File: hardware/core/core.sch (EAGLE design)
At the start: 529 parts, among them IC1 MAX481CSA, IC10 MAX481CSA, IC11 MAX481CSA, IC12 MAX481CSA, IC13 MAX481CSA, IC14 MAX481CSA, IC15 MAX481CSA, IC16 MAX481CSA, IC17 MAX481CSA, IC18 MAX481CSA, IC19 MAX481CSA, IC2 LD117AS12TR, IC20 MAX481CSA, IC21 MAX481CSA, IC22 LD117AS12TR, IC23 LD117AS12TR, IC3 MAX481CSA, IC4 MAX481CSA, IC5 MAX481CSA, IC6 MAX481CSA, IC7 MAX481CSA, IC8 MAX481CSA, IC9 MAX481CSA

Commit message: Update phoenix connectors & add JLC_ROTATION
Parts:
- added D100, D101, D102, D103, D104, D105, D106, D107, D108, D109, D110, D111, D112, D113, D114, D95, D96, D97, D98, D99: D_B5819W-SL_CHANGJ_SOD123, JLC PCB Basic Parts_loc:D_B5819W-SL_CHANGJ_SOD123
- POWER_IN: device con-phoenix-508:MKDSN1,5/4-5,08 -> con-phoenix-508-jm:MKDSN1,5/4-5,08
- R132: value R_1.8K_0603 -> R_1K_0603; device JLC PCB Basic Parts_loc:R_1.8K_0603 -> JLC PCB Basic Parts_loc:R_1K_0603
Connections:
- new net N$325: D95.C, STAR_1.6
- new net N$326: D97.C, STAR_3.6
- new net N$327: D96.A, R55.2
- new net N$328: D96.C, STAR_2.6
- new net N$329: D100.A, R59.2
- new net N$330: D100.C, STAR_6.6
- new net N$331: D99.A, R58.2
- new net N$332: D99.C, STAR_5.6
- new net N$333: D110.A, R85.2
- new net N$334: D110.C, STAR_15.6
- new net N$335: D109.A, R84.2
- new net N$336: D109.C, STAR_14.6
- new net N$337: D105.A, R103.2
- new net N$338: D105.C, STAR_17.6
- new net N$339: D112.A, R104.2
- new net N$340: D112.C, STAR_18.6
- new net N$341: D113.A, R105.2
- new net N$342: D113.C, STAR_19.6
- new net N$343: D114.A, R106.2
- new net N$344: D114.C, STAR_20.6
- net N$10: now also D102.A, R61.2; no longer R58.2, STAR_5.6
- net N$104: now also D108.A, R65.2; no longer R104.2, STAR_18.6
- net N$105: now also D108.C, STAR_12.6; no longer R105.2, STAR_19.6
- net N$106: now also D111.A, R86.2; no longer R106.2, STAR_20.6
- net N$107: now also D111.C, STAR_16.6; no longer R103.2, STAR_17.6
- net N$15: now also D102.C, STAR_8.6; no longer R59.2, STAR_6.6
- net N$16: now also D101.A; no longer STAR_7.6
- net N$17: now also D101.C, STAR_7.6; no longer R61.2, STAR_8.6
- net N$18: now also D103.A, R62.2; no longer R65.2, STAR_12.6
- net N$19: now also D103.C, STAR_9.6; no longer R64.2, STAR_11.6
- net N$2: now also D98.A, R57.2; no longer R55.2, STAR_2.6
- net N$24: now also D104.A, R83.2; no longer R63.2, STAR_10.6
- net N$25: now also D104.C, STAR_13.6; no longer R62.2, STAR_9.6
- net N$7: now also D98.C, STAR_4.6; no longer R56.2, STAR_3.6
- net N$72: now also D106.A, R63.2; no longer R84.2, STAR_14.6
- net N$73: now also D106.C, STAR_10.6; no longer R85.2, STAR_15.6
- net N$74: now also D107.A, R64.2; no longer R86.2, STAR_16.6
- net N$75: now also D107.C, STAR_11.6; no longer R83.2, STAR_13.6
- net N$8: now also D97.A, R56.2; no longer R57.2, STAR_4.6
- net N$9: now also D95.A; no longer STAR_1.6

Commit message: Replaced output resistor with 68 ohm (part c27592)
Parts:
- R103, R104, R105, R106, R140, R141, R142, R143, R144, R145, R146, R147, R148, R149, R150, R151, R152, R153, R154, R155, R156, R157, R158, R159, R160, R161, R162, R163, R164, R165, R166, R167, R168, R169, R170, R171, R172, R173, R174, R175, R176, R177, R178, R179, R180, R181, R182, R183, R184, R185, R186, R187, R188, R189, R190, R191, R192, R193, R194, R195, R196, R197, R198, R199, R200, R201, R202, R203, R204, R205, R206, R207, R208, R209, R210, R211, R212, R213, R214, R215, R216, R217, R218, R219, R54, R55, R56, R57, R58, R59, R60, R61, R62, R63, R64, R65, R83, R84, R85, R86: LCSC_PART C25804 -> c27592

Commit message: Add TVS and change led resistors to 1k
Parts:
- removed I2C_1: (no value), pinhead:PINHD-1X4
- removed ULN10, ULN11, ULN12, ULN3, ULN4, ULN5, ULN6, ULN7, ULN8, ULN9: (no value), SparkFun-IC-Special-Function:ULN2803SOICW
- added D115, D116, D117, D118, D119, D120, D121, D122, D123, D124, D125, D126, D127, D128, D129, D130, D131, D132, D133, D134, D135, D136, D137, D138, D139, D140, D141, D142, D143, D144, D145, D146, D147, D148, D149, D150, D151, D152, D153, D154, D155, D156, D157, D158, D159, D160, D161, D162, D163, D164, D165, D166, D167, D168, D169, D170, D171, D172, D173, D174, D175, D176, D177, D178, D179, D180, D181, D182, D183, D184, D185, D186, D187, D188, D189, D190, D191, D192, D193, D194, D195: SMBJ8.0CA, SMBJ8.0CA:SMBJ8.0CA
- added R226, R227, R228, R229, R230, R231, R232, R233, R234, R235, R236, R237, R238, R239, R240, R241, R242, R243, R244, R245, R246, R247, R248, R249, R250, R251, R252, R253, R254, R255, R256, R257, R258, R259, R260, R261, R262, R263, R264, R265, R266, R267, R268, R269, R270, R271, R272, R273, R274, R275, R276, R277, R278, R279, R280, R281, R282, R283, R284, R285, R286, R287, R288, R289, R290, R291, R292, R293, R294, R295, R296, R297, R298, R299, R300, R301, R302, R303, R304, R305: 68, rcl:R-US_R0603
- R10, R100, R101, R102, R11, R12, R13, R14, R15, R16, R17, R18, R19, R20, R21, R22, R23, R24, R25, R28, R29, R3, R30, R31, R32, R33, R34, R35, R36, R37, R38, R39, R4, R40, R41, R42, R43, R44, R45, R46, R47, R48, R49, R5, R50, R51, R52, R53, R6, R66, R69, R7, R70, R71, R72, R73, R74, R75, R76, R77, R78, R79, R8, R80, R81, R82, R87, R88, R89, R9, R90, R91, R92, R93, R94, R95, R96, R97, R98, R99: value 10k -> 1k; LCSC_PART C25804 -> C21190
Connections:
- new net N$345: C45.1, D123.2, R11.1, R151.1, R234.2
- net +12V: no longer ULN10.10, ULN11.10, ULN12.10, ULN3.10, ULN4.10, ULN5.10, ULN6.10, ULN7.10, ULN8.10, ULN9.10
- net +3V3: no longer I2C_1.1
- net +5V: no longer D1.A, D10.A, D11.A, D12.A, D13.A, D14.A, D15.A, D16.A, D17.A, D18.A, D19.A, D2.A, D20.A, D21.A, D22.A, D23.A, D24.A, D25.A, D26.A, D27.A, D28.A, D29.A, D3.A, D30.A, D31.A, D32.A, D33.A, D34.A, D35.A, D36.A, D37.A, D38.A, D39.A, D4.A, D40.A, D41.A, D42.A, D43.A, D44.A, D45.A, D46.A, D47.A, D48.A, D49.A, D5.A, D50.A, D51.A, D52.A, D53.A, D54.A, D55.A, D56.A, D57.A, D58.A, D59.A, D6.A, D60.A, D61.A, D62.A, D63.A, D64.A, D65.A, D66.A, D67.A, D68.A, D69.A, D7.A, D70.A, D71.A, D72.A, D73.A, D74.A, D75.A, D76.A, D77.A, D78.A, D79.A, D8.A, D80.A, D9.A
- net 21/SDA: no longer I2C_1.4
- net 22/SCL: no longer I2C_1.3
- net A0: now also R226.1; no longer ULN3.8
- net A1: now also R227.1; no longer ULN3.7
- net A10: now also R236.1; no longer ULN4.6
- net A11: now also R237.1; no longer ULN4.5
- net A12: now also R238.1; no longer ULN4.4
- net A13: now also R239.1; no longer ULN4.3
- net A14: now also R240.1; no longer ULN4.2
- net A15: now also R241.1; no longer ULN4.1
- net A2: now also R228.1; no longer ULN3.6
- net A3: now also R229.1; no longer ULN3.5
- net A4: now also R230.1; no longer ULN3.4
- net A5: now also R231.1; no longer ULN3.3
- net A6: now also R232.1; no longer ULN3.2
- net A7: now also R233.1; no longer ULN3.1
- net A8: now also R234.1; no longer ULN4.8
- net A9: now also R235.1; no longer ULN4.7
- net B0: now also R242.1; no longer ULN5.8
- net B1: now also R243.1; no longer ULN5.7
- net B10: now also R252.1; no longer ULN6.6
- net B11: now also R253.1; no longer ULN6.5
- net B12: now also R254.1; no longer ULN6.4
- net B13: now also R255.1; no longer ULN6.3
- net B14: now also R256.1; no longer ULN6.2
- net B15: now also R257.1; no longer ULN6.1
- net B2: now also R244.1; no longer ULN5.6
- net B3: now also R245.1; no longer ULN5.5
- net B4: now also R246.1; no longer ULN5.4
- net B5: now also R247.1; no longer ULN5.3
- net B6: now also R248.1; no longer ULN5.2
- net B7: now also R249.1; no longer ULN5.1
- net B8: now also R250.1; no longer ULN6.8
- net B9: now also R251.1; no longer ULN6.7
- net C0: now also R258.1; no longer ULN7.8
- net C1: now also R259.1; no longer ULN7.7
- net C10: now also R268.1; no longer ULN8.6
- net C11: now also R269.1; no longer ULN8.5
- net C12: now also R270.1; no longer ULN8.4
- net C13: now also R271.1; no longer ULN8.3
- net C14: now also R272.1; no longer ULN8.2
- net C15: now also R273.1; no longer ULN8.1
- net C2: now also R260.1; no longer ULN7.6
- net C3: now also R261.1; no longer ULN7.5
- net C4: now also R262.1; no longer ULN7.4
- net C5: now also R263.1; no longer ULN7.3
- net C6: now also R264.1; no longer ULN7.2
- net C7: now also R265.1; no longer ULN7.1
- net C8: now also R266.1; no longer ULN8.8
- net C9: now also R267.1; no longer ULN8.7
- net D0: now also R274.1; no longer ULN9.8
- net D1: now also R275.1; no longer ULN9.7
- net D10: now also R284.1; no longer ULN10.6
- net D11: now also R285.1; no longer ULN10.5
- net D12: now also R286.1; no longer ULN10.4
- net D13: now also R287.1; no longer ULN10.3
- net D14: now also R288.1; no longer ULN10.2
- net D15: now also R289.1; no longer ULN10.1
- net D2: now also R276.1; no longer ULN9.6
- net D3: now also R277.1; no longer ULN9.5
- net D4: now also R278.1; no longer ULN9.4
- net D5: now also R279.1; no longer ULN9.3
- net D6: now also R280.1; no longer ULN9.2
- net D7: now also R281.1; no longer ULN9.1
- net D8: now also R282.1; no longer ULN10.8
- net D9: now also R283.1; no longer ULN10.7
- net E0: now also R290.1; no longer ULN11.8
- net E1: now also R291.1; no longer ULN11.7
- net E10: now also R300.1; no longer ULN12.6
- net E11: now also R301.1; no longer ULN12.5
- net E12: now also R302.1; no longer ULN12.4
- net E13: now also R303.1; no longer ULN12.3
- net E14: now also R304.1; no longer ULN12.2
- net E15: now also R305.1; no longer ULN12.1
- net E2: now also R292.1; no longer ULN11.6
- net E3: now also R293.1; no longer ULN11.5
- net E4: now also R294.1; no longer ULN11.4
- net E5: now also R295.1; no longer ULN11.3
- net E6: now also R296.1; no longer ULN11.2
- net E7: now also R297.1; no longer ULN11.1
- net E8: now also R298.1; no longer ULN12.8
- net E9: now also R299.1; no longer ULN12.7
- net GND: now also D10.C, D11.C, D115.1, D116.1, D117.1, D118.1, D119.1, D12.C, D120.1, D121.1, D122.1, D123.1, D124.1, D125.1, D126.1, D127.1, D128.1, D129.1, D13.C, D130.1, D131.1, D132.1, D133.1, D134.1, D135.1, D136.1, D137.1, D138.1, D139.1, D14.C, D140.1, D141.1, D142.1, D143.1, D144.1, D145.1, D146.1, D147.1, D148.1, D149.1, D15.C, D150.1, D151.1, D152.1, D153.1, D154.1, D155.1, D156.1, D157.1, D158.1, D159.1, D16.C, D160.1, D161.1, D162.1, D163.1, D164.1, D165.1, D166.1, D167.1, D168.1, D169.1, D17.C, D170.1, D171.1, D172.1, D173.1, D174.1, D175.1, D176.1, D177.1, D178.1, D179.1, D18.C, D180.1, D181.1, D182.1, D183.1, D184.1, D185.1, D186.1, D187.1, D188.1, D189.1, D19.C, D190.1, D191.1, D192.1, D193.1, D194.1, D195.1, D2.C, D20.C, D21.C, D22.C, D23.C, D24.C, D25.C, D26.C, D27.C, D28.C, D29.C, D3.C, D30.C, D31.C, D32.C, D33.C, D34.C, D35.C, D36.C, D37.C, D38.C, D39.C, D4.C, D40.C, D41.C, D42.C, D43.C, D44.C, D45.C, D46.C, D47.C, D48.C, D49.C, D5.C, D57.C, D58.C, D59.C, D6.C, D60.C, D61.C, D62.C, D63.C, D64.C, D65.C, D66.C, D67.C, D68.C, D69.C, D7.C, D70.C, D71.C, D72.C, D73.C, D74.C, D75.C, D76.C, D77.C, D78.C, D79.C, D8.C, D80.C, D9.C; no longer I2C_1.2, ULN10.9, ULN11.9, ULN12.9, ULN3.9, ULN4.9, ULN5.9, ULN6.9, ULN7.9, ULN8.9, ULN9.9
- net N$100: now also D69.A, R91.2; no longer D77.C, R99.2
- net N$101: now also D70.A, R92.2; no longer D78.C, R100.2
- net N$102: now also D71.A, R93.2; no longer D79.C, R101.2
- net N$103: now also D72.A, R94.2; no longer D80.C, R102.2
- net N$11: now also D6.A; no longer D6.C
- net N$12: now also D7.A; no longer D7.C
- net N$13: now also D8.A; no longer D8.C
- net N$14: now also D9.A; no longer D9.C
- net N$160: now also D116.2, R226.2; no longer ULN3.11
- net N$161: now also D115.2, R227.2; no longer ULN3.12
- net N$162: now also D117.2, R228.2; no longer ULN3.13
- net N$163: now also D118.2, R229.2; no longer ULN3.14
- net N$164: now also D122.2, R233.2; no longer ULN3.18
- net N$165: now also D121.2, R232.2; no longer ULN3.17
- net N$166: now also D120.2, R231.2; no longer ULN3.16
- net N$167: now also D119.2, R230.2; no longer ULN3.15
- net N$184: now also D49.A, R52.2; no longer C45.1, R11.1, R151.1, ULN4.11
- net N$185: now also D124.2, R235.2; no longer ULN4.12
- net N$186: now also D125.2, R236.2; no longer ULN4.13
- net N$187: now also D126.2, R237.2; no longer ULN4.14
- net N$188: now also D130.2, R241.2; no longer ULN4.18
- net N$189: now also D129.2, R240.2; no longer ULN4.17
- net N$190: now also D128.2, R239.2; no longer ULN4.16
- net N$191: now also D127.2, R238.2; no longer ULN4.15
- net N$192: now also D131.2, R242.2; no longer ULN5.11
- net N$193: now also D134.2, R245.2; no longer ULN5.14
- net N$194: now also D133.2, R244.2; no longer ULN5.13
- net N$195: now also D132.2, R243.2; no longer ULN5.12
- net N$196: now also D138.2, R249.2; no longer ULN5.18
- net N$197: now also D137.2, R248.2; no longer ULN5.17
- net N$198: now also D136.2, R247.2; no longer ULN5.16
- net N$199: now also D135.2, R246.2; no longer ULN5.15
- net N$20: now also D14.A, R15.2; no longer D10.C, R11.2
- net N$21: now also D15.A, R16.2; no longer D11.C, R12.2
- net N$216: now also D139.2, R250.2; no longer ULN6.11
- net N$217: now also D140.2, R251.2; no longer ULN6.12
- net N$218: now also D141.2, R252.2; no longer ULN6.13
- net N$219: now also D142.2, R253.2; no longer ULN6.14
- net N$22: now also D16.A, R17.2; no longer D12.C, R13.2
- net N$220: now also D146.2, R257.2; no longer ULN6.18
- net N$221: now also D145.2, R256.2; no longer ULN6.17
- net N$222: now also D144.2, R255.2; no longer ULN6.16
- net N$223: now also D143.2, R254.2; no longer ULN6.15
- net N$23: now also D17.A, R18.2; no longer D13.C, R14.2
- net N$240: now also D147.2, R258.2; no longer ULN7.11
- net N$241: now also D148.2, R259.2; no longer ULN7.12
- net N$242: now also D149.2, R260.2; no longer ULN7.13
- net N$243: now also D150.2, R261.2; no longer ULN7.14
- net N$245: now also D153.2, R264.2; no longer ULN7.17
- net N$246: now also D152.2, R263.2; no longer ULN7.16
- net N$247: now also D151.2, R262.2; no longer ULN7.15
- net N$248: now also D155.2, R266.2; no longer ULN8.11
- net N$249: now also D156.2, R267.2; no longer ULN8.12
- net N$250: now also D157.2, R268.2; no longer ULN8.13
- net N$251: now also D158.2, R269.2; no longer ULN8.14
- net N$252: now also D154.2, R265.2; no longer ULN7.18
- net N$253: now also D161.2, R272.2; no longer ULN8.17
- net N$254: now also D160.2, R271.2; no longer ULN8.16
- net N$255: now also D159.2, R270.2; no longer ULN8.15
- net N$26: now also D56.A, R74.2; no longer D1.C, R53.2
- net N$260: now also D162.2, R273.2; no longer ULN8.18
- net N$27: now also D55.A, R73.2; no longer D50.C, R66.2
- net N$28: now also D13.A, R14.2; no longer D14.C, R15.2
- net N$288: now also D172.2, R282.2; no longer ULN10.11
- net N$289: now also D173.2, R283.2; no longer ULN10.12
- net N$29: now also D12.A, R13.2; no longer D15.C, R16.2
- net N$290: now also D174.2, R284.2; no longer ULN10.13
- net N$291: now also D175.2, R285.2; no longer ULN10.14
- net N$292: now also D179.2, R289.2; no longer ULN10.18
- net N$293: now also D178.2, R288.2; no longer ULN10.17
- net N$294: now also D177.2, R287.2; no longer ULN10.16
- net N$295: now also D176.2, R286.2; no longer ULN10.15
- net N$296: now also D163.2, R274.2; no longer ULN9.11
- net N$297: now also D164.2, R275.2; no longer ULN9.12
- net N$298: now also D165.2, R276.2; no longer ULN9.13
- net N$299: now also D166.2, R277.2; no longer ULN9.14
- net N$3: now also D2.A; no longer D2.C
- net N$30: now also D11.A, R12.2; no longer D16.C, R17.2
- net N$300: now also D170.2, R281.2; no longer ULN9.18
- net N$301: now also D169.2, R280.2; no longer ULN9.17
- net N$302: now also D168.2, R279.2; no longer ULN9.16
- net N$303: now also D167.2, R278.2; no longer ULN9.15
- net N$304: now also D180.2, R290.2; no longer ULN11.11
- net N$305: now also D181.2, R291.2; no longer ULN11.12
- net N$306: now also D182.2, R292.2; no longer ULN11.13
- net N$307: now also D183.2, R293.2; no longer ULN11.14
- net N$308: now also D187.2, R297.2; no longer ULN11.18
- net N$309: now also D186.2, R296.2; no longer ULN11.17
- net N$31: now also D10.A, R11.2; no longer D17.C, R18.2
- net N$310: now also D185.2, R295.2; no longer ULN11.16
- net N$311: now also D184.2, R294.2; no longer ULN11.15
- net N$312: now also D188.2, R298.2; no longer ULN12.11
- net N$313: now also D189.2, R299.2; no longer ULN12.12
- net N$314: now also D190.2, R300.2; no longer ULN12.13
- net N$315: now also D191.2, R301.2; no longer ULN12.14
- net N$316: now also D195.2, R305.2; no longer ULN12.18
- net N$317: now also D194.2, R304.2; no longer ULN12.17
- net N$318: now also D193.2, R303.2; no longer ULN12.16
- net N$319: now also D192.2, R302.2; no longer ULN12.15
- net N$32: now also D54.A, R72.2; no longer D51.C, R69.2
- net N$33: now also D53.A, R71.2; no longer D52.C, R70.2
- net N$34: now also D80.A, R102.2; no longer D65.C, R87.2
- net N$35: now also D1.A, R53.2; no longer D53.C, R71.2
- net N$36: now also D25.A, R28.2; no longer D18.C, R19.2
- net N$37: now also D24.A, R25.2; no longer D19.C, R20.2
- net N$38: now also D23.A, R24.2; no longer D20.C, R21.2
- net N$39: now also D22.A, R23.2; no longer D21.C, R22.2
- net N$4: now also D3.A; no longer D3.C
- net N$40: now also D50.A, R66.2; no longer D54.C, R72.2
- net N$41: now also D51.A, R69.2; no longer D55.C, R73.2
- net N$42: now also D52.A, R70.2; no longer D56.C, R74.2
- net N$43: now also D61.A, R79.2; no longer D57.C, R75.2
- net N$44: now also D21.A, R22.2; no longer D22.C, R23.2
- net N$45: now also D20.A, R21.2; no longer D23.C, R24.2
- net N$46: now also D19.A, R20.2; no longer D24.C, R25.2
- net N$47: now also D18.A, R19.2; no longer D25.C, R28.2
- net N$48: now also D62.A, R80.2; no longer D58.C, R76.2
- net N$49: now also D63.A, R81.2; no longer D59.C, R77.2
- net N$5: now also D4.A; no longer D4.C
- net N$50: now also D64.A, R82.2; no longer D60.C, R78.2
- net N$52: now also D26.A; no longer D26.C
- net N$53: now also D27.A; no longer D27.C
- net N$54: now also D28.A; no longer D28.C
- net N$55: now also D29.A; no longer D29.C
- net N$6: now also D5.A; no longer D5.C
- net N$60: now also D30.A; no longer D30.C
- net N$61: now also D31.A; no longer D31.C
- net N$62: now also D32.A; no longer D32.C
- net N$63: now also D33.A; no longer D33.C
- net N$64: now also D57.A, R75.2; no longer D61.C, R79.2
- net N$65: now also D58.A, R76.2; no longer D62.C, R80.2
- net N$66: now also D59.A, R77.2; no longer D63.C, R81.2
- net N$67: now also D60.A, R78.2; no longer D64.C, R82.2
- net N$68: now also D34.A; no longer D34.C
- net N$69: now also D35.A; no longer D35.C
- net N$70: now also D36.A; no longer D36.C
- net N$71: now also D37.A; no longer D37.C
- net N$76: now also D38.A; no longer D38.C
- net N$77: now also D39.A; no longer D39.C
- net N$78: now also D40.A; no longer D40.C
- net N$79: now also D41.A; no longer D41.C
- net N$80: now also D79.A, R101.2; no longer D66.C, R88.2
- net N$81: now also D78.A, R100.2; no longer D67.C, R89.2
- net N$82: now also D77.A, R99.2; no longer D68.C, R90.2
- net N$83: now also D76.A, R98.2; no longer D69.C, R91.2
- net N$84: now also D1.C, D50.C, D51.C, D52.C, D53.C, D54.C, D55.C, D56.C; no longer D42.C, R45.2
- net N$85: now also D42.A, R45.2; no longer D43.C, R46.2
- net N$86: now also D43.A, R46.2; no longer D44.C, R47.2
- net N$87: now also D44.A, R47.2; no longer D45.C, R48.2
- net N$88: now also D75.A, R97.2; no longer D70.C, R92.2
- net N$90: now also D74.A, R96.2; no longer D71.C, R93.2
- net N$91: now also D73.A, R95.2; no longer D72.C, R94.2
- net N$92: now also D65.A, R87.2; no longer D73.C, R95.2
- net N$93: now also D45.A, R48.2; no longer D46.C, R49.2
- net N$94: now also D46.A, R49.2; no longer D47.C, R50.2
- net N$95: now also D47.A, R50.2; no longer D48.C, R51.2
- net N$96: now also D48.A, R51.2; no longer D49.C, R52.2
- net N$97: now also D66.A, R88.2; no longer D74.C, R96.2
- net N$98: now also D67.A, R89.2; no longer D75.C, R97.2
- net N$99: now also D68.A, R90.2; no longer D76.C, R98.2
- net STAR_ENABLE: now also D171.2
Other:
- moved on the sheet: ACCESSORY, C100, C101, C102, C103, C104, C105, C106, C107, C108, C109, C110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

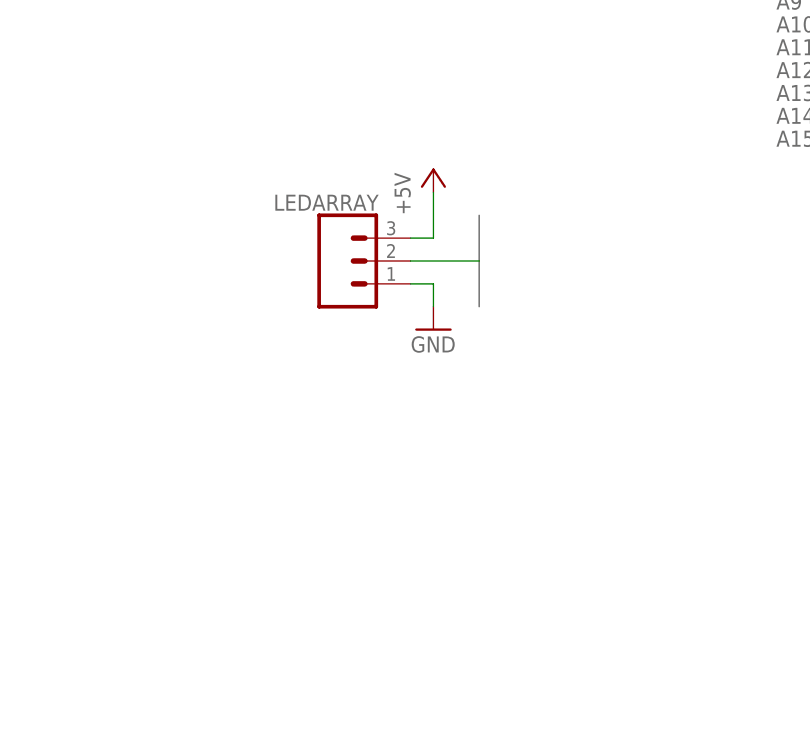
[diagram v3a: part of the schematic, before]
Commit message: misc board updates
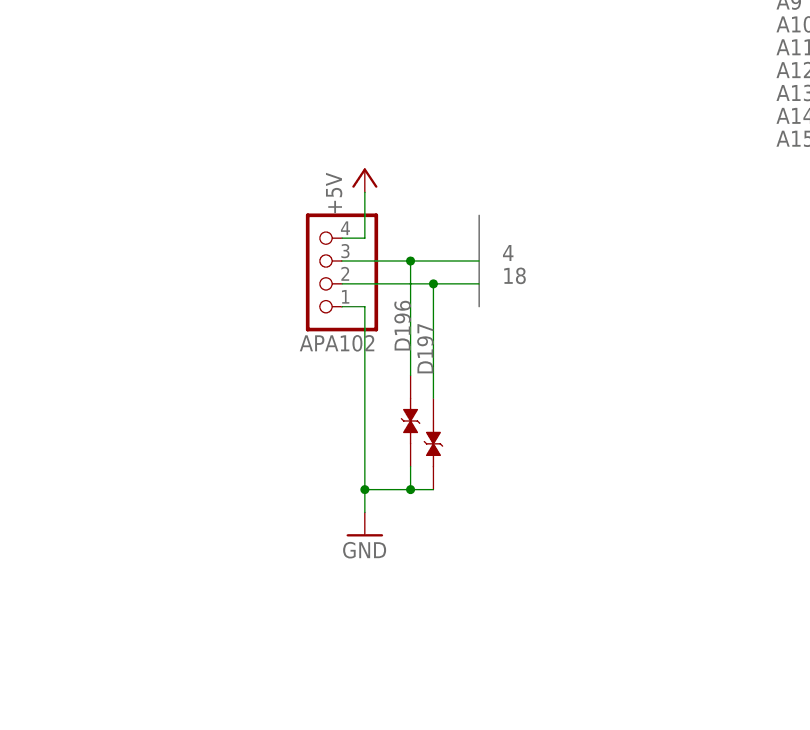
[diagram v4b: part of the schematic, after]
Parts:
- removed LEDARRAY: (no value), SparkFun-Connectors:CONN_03LONGPADS
- added APA102: (no value), pinhead:PINHD-1X4
- added D196, D197: SMBJ8.0CA, SMBJ8.0CA:SMBJ8.0CA
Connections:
- net +5V: now also APA102.4; no longer LEDARRAY.3
- net 18: now also APA102.2, D197.2
- net 4: now also APA102.3, D196.2; no longer LEDARRAY.2
- net GND: now also APA102.1, D196.1, D197.1; no longer LEDARRAY.1
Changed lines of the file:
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@@
 <part name="GND96" library="supply1" library_urn="urn:adsk.eagle:library:371" deviceset="GND" device=""/>
 <part name="+3V47" library="supply1" library_urn="urn:adsk.eagle:library:371" deviceset="+3V3" device=""/>
-<part name="LEDARRAY" library="SparkFun-Connectors" library_urn="urn:adsk.eagle:library:513" deviceset="CONN_03" device="LONGPADS" package3d_urn="urn:adsk.eagle:package:38068/1"/>
 <part name="GND95" library="supply1" library_urn="urn:adsk.eagle:library:371" deviceset="GND" device=""/>
 <part name="P+4" library="supply1" library_urn="urn:adsk.eagle:library:371" deviceset="+5V" device=""/>
@@
 <part name="GND125" library="supply1" library_urn="urn:adsk.eagle:library:371" deviceset="GND" device=""/>
 <part name="GND126" library="supply1" library_urn="urn:adsk.eagle:library:371" deviceset="GND" device=""/>
+<part name="APA102" library="pinhead" library_urn="urn:adsk.eagle:library:325" deviceset="PINHD-1X4" device="" package3d_urn="urn:adsk.eagle:package:22407/2"/>
+<part name="D196" library="SMBJ8.0CA" library_urn="urn:adsk.eagle:library:39221370" deviceset="SMBJ8.0CA" device="" package3d_urn="urn:adsk.eagle:package:39221373/1">
+<attribute name="DESCRIPTION" value="600 Watt TVS 5.0v working, 9v clamp"/>
+<attribute name="LCSC_PART" value="C78757"/>
+</part>
+<part name="D197" library="SMBJ8.0CA" library_urn="urn:adsk.eagle:library:39221370" deviceset="SMBJ8.0CA" device="" package3d_urn="urn:adsk.eagle:package:39221373/1">
+<attribute name="DESCRIPTION" value="600 Watt TVS 5.0v working, 9v clamp"/>
+<attribute name="LCSC_PART" value="C78757"/>
+</part>
 </parts>
 <sheets>
@@
 <attribute name="VALUE" x="848.36" y="-68.58" size="1.778" layer="96" rot="R90"/>
 </instance>
-<instance part="LEDARRAY" gate="J$1" x="304.8" y="-71.12" smashed="yes">
-<attribute name="VALUE" x="302.26" y="-78.486" size="1.778" layer="96" font="vector"/>
-<attribute name="NAME" x="297.18" y="-65.532" size="1.778" layer="95" font="vector"/>
-</instance>
-<instance part="GND95" gate="1" x="314.96" y="-78.74" smashed="yes">
-<attribute name="VALUE" x="312.42" y="-81.28" size="1.778" layer="96"/>
+<instance part="GND95" gate="1" x="307.34" y="-101.6" smashed="yes">
+<attribute name="VALUE" x="304.8" y="-104.14" size="1.778" layer="96"/>
 </instance>
-<instance part="P+4" gate="1" x="314.96" y="-60.96" smashed="yes">
-<attribute name="VALUE" x="312.42" y="-66.04" size="1.778" layer="96" rot="R90"/>
+<instance part="P+4" gate="1" x="307.34" y="-60.96" smashed="yes">
+<attribute name="VALUE" x="304.8" y="-66.04" size="1.778" layer="96" rot="R90"/>
 </instance>
 <instance part="ACCESSORY" gate="A" x="129.54" y="-15.24" smashed="yes">
@@
 <attribute name="VALUE" x="1198.88" y="182.88" size="1.778" layer="96"/>
 </instance>
+<instance part="APA102" gate="A" x="302.26" y="-71.12" smashed="yes" rot="R180">
+<attribute name="NAME" x="308.61" y="-79.375" size="1.778" layer="95" rot="R180"/>
+<attribute name="VALUE" x="308.61" y="-63.5" size="1.778" layer="96" rot="R180"/>
+</instance>
+<instance part="D196" gate="G$1" x="312.42" y="-88.9" smashed="yes" rot="R90">
+<attribute name="NAME" x="312.42" y="-81.28" size="1.778" layer="95" rot="R90"/>
+<attribute name="LCSC_PART" x="312.42" y="-88.9" size="1.778" layer="96" rot="R90" display="off"/>
+</instance>
+<instance part="D197" gate="G$1" x="314.96" y="-91.44" smashed="yes" rot="R90">
+<attribute name="NAME" x="314.96" y="-83.82" size="1.778" layer="95" rot="R90"/>
+<attribute name="LCSC_PART" x="314.96" y="-91.44" size="1.778" layer="96" rot="R90" display="off"/>
+</instance>
 </instances>
 <busses>
@@
 <segment>
 <pinref part="GND95" gate="1" pin="GND"/>
-<pinref part="LEDARRAY" gate="J$1" pin="1"/>
-<wire x1="314.96" y1="-76.2" x2="314.96" y2="-73.66" width="0.1524" layer="91"/>
-<wire x1="314.96" y1="-73.66" x2="312.42" y2="-73.66" width="0.1524" layer="91"/>
+<wire x1="307.34" y1="-99.06" x2="307.34" y2="-96.52" width="0.1524" layer="91"/>
+<wire x1="307.34" y1="-96.52" x2="307.34" y2="-76.2" width="0.1524" layer="91"/>
+<wire x1="307.34" y1="-76.2" x2="304.8" y2="-76.2" width="0.1524" layer="91"/>
+<pinref part="APA102" gate="A" pin="1"/>
+<pinref part="D197" gate="G$1" pin="1"/>
+<wire x1="314.96" y1="-96.52" x2="312.42" y2="-96.52" width="0.1524" layer="91"/>
+<junction x="307.34" y="-96.52"/>
+<pinref part="D196" gate="G$1" pin="1"/>
+<wire x1="312.42" y1="-96.52" x2="307.34" y2="-96.52" width="0.1524" layer="91"/>
+<wire x1="312.42" y1="-93.98" x2="312.42" y2="-96.52" width="0.1524" layer="91"/>
+<junction x="312.42" y="-96.52"/>
 </segment>
 <segment>
@@
 </segment>
 <segment>
-<pinref part="LEDARRAY" gate="J$1" pin="3"/>
 <pinref part="P+4" gate="1" pin="+5V"/>
-<wire x1="312.42" y1="-68.58" x2="314.96" y2="-68.58" width="0.1524" layer="91"/>
-<wire x1="314.96" y1="-68.58" x2="314.96" y2="-63.5" width="0.1524" layer="91"/>
+<wire x1="304.8" y1="-68.58" x2="307.34" y2="-68.58" width="0.1524" layer="91"/>
+<wire x1="307.34" y1="-68.58" x2="307.34" y2="-63.5" width="0.1524" layer="91"/>
+<pinref part="APA102" gate="A" pin="4"/>
 </segment>
 <segment>
@@
 <label x="139.7" y="104.14" size="1.778" layer="95"/>
 </segment>
+<segment>
+<pinref part="APA102" gate="A" pin="2"/>
+<wire x1="320.04" y1="-73.66" x2="314.96" y2="-73.66" width="0.1524" layer="91"/>
+<label x="322.58" y="-73.66" size="1.778" layer="95"/>
+<pinref part="D197" gate="G$1" pin="2"/>
+<wire x1="314.96" y1="-73.66" x2="304.8" y2="-73.66" width="0.1524" layer="91"/>
+<wire x1="314.96" y1="-86.36" x2="314.96" y2="-73.66" width="0.1524" layer="91"/>
+<junction x="314.96" y="-73.66"/>
+</segment>
 </net>
 <net name="5" class="0">
@@
 </segment>
 <segment>
-<pinref part="LEDARRAY" gate="J$1" pin="2"/>
 <wire x1="320.04" y1="-71.12" x2="312.42" y2="-71.12" width="0.1524" layer="91"/>
+<label x="322.58" y="-71.12" size="1.778" layer="95"/>
+<pinref part="APA102" gate="A" pin="3"/>
+<pinref part="D196" gate="G$1" pin="2"/>
+<wire x1="312.42" y1="-71.12" x2="304.8" y2="-71.12" width="0.1524" layer="91"/>
+<wire x1="312.42" y1="-83.82" x2="312.42" y2="-71.12" width="0.1524" layer="91"/>
+<junction x="312.42" y="-71.12"/>
 </segment>
 </net>
